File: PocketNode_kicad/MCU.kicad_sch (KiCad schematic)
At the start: 10 parts, among them U3 ESP32-S3-WROOM-1-N16R8

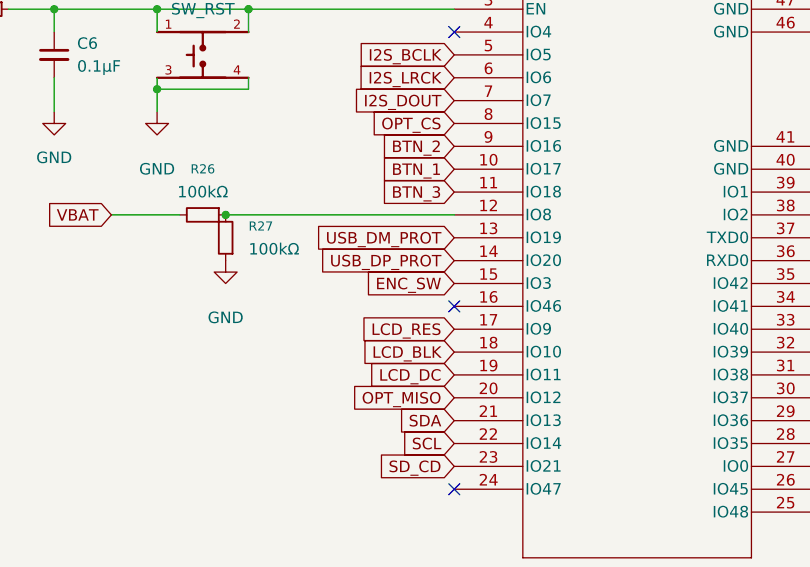
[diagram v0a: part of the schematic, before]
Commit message: update
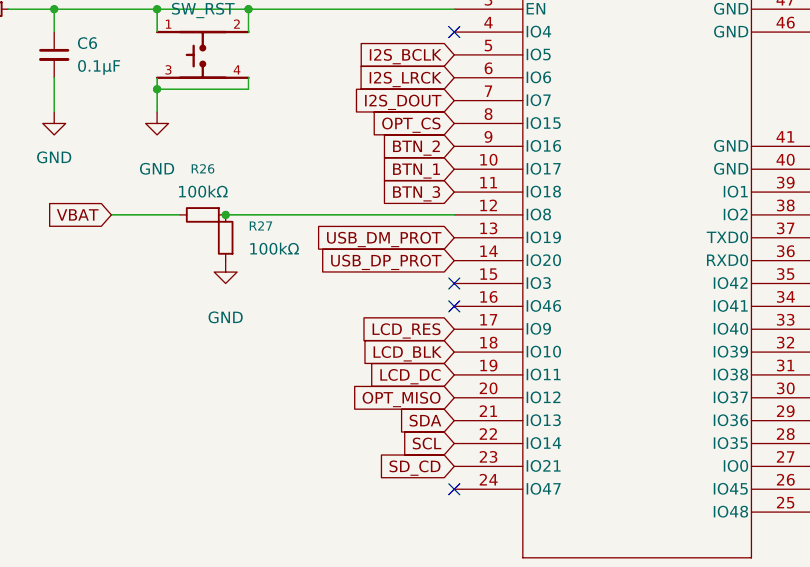
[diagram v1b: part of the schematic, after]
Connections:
- net ENC_SW: no longer names the net of U3.15 (IO3)
- no-connect marks 9 -> 10
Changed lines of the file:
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@@
+	)
+	(no_connect
+		(at 128.27 64.77)
 	)
 	(no_connect
@@
 			(effects
 				(font
-					(size 1.27 1.27)
-				)
-				(justify right)
-				(hide yes)
-			)
-		)
-	)
-	(global_label "ENC_SW"
-		(shape input)
-		(at 128.27 64.77 180)
-		(fields_autoplaced yes)
-		(effects
-			(font
-				(size 1.27 1.27)
-			)
-			(justify right)
-		)
-		(property "Intersheetrefs" "${INTERSHEET_REFS}"
-			(at 117.9068 64.77 0)
-			(effects
-				(font
